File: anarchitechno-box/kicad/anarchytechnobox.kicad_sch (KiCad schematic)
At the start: 19 parts, among them J1 Conn_01x02, Q1 IRLZ44N, Q2 IRFS4310Z, U1 TC4426xOA, U2 ADuM1200AR, U4 LM7812_TO220, U5 L7805, U6 TME-0503S

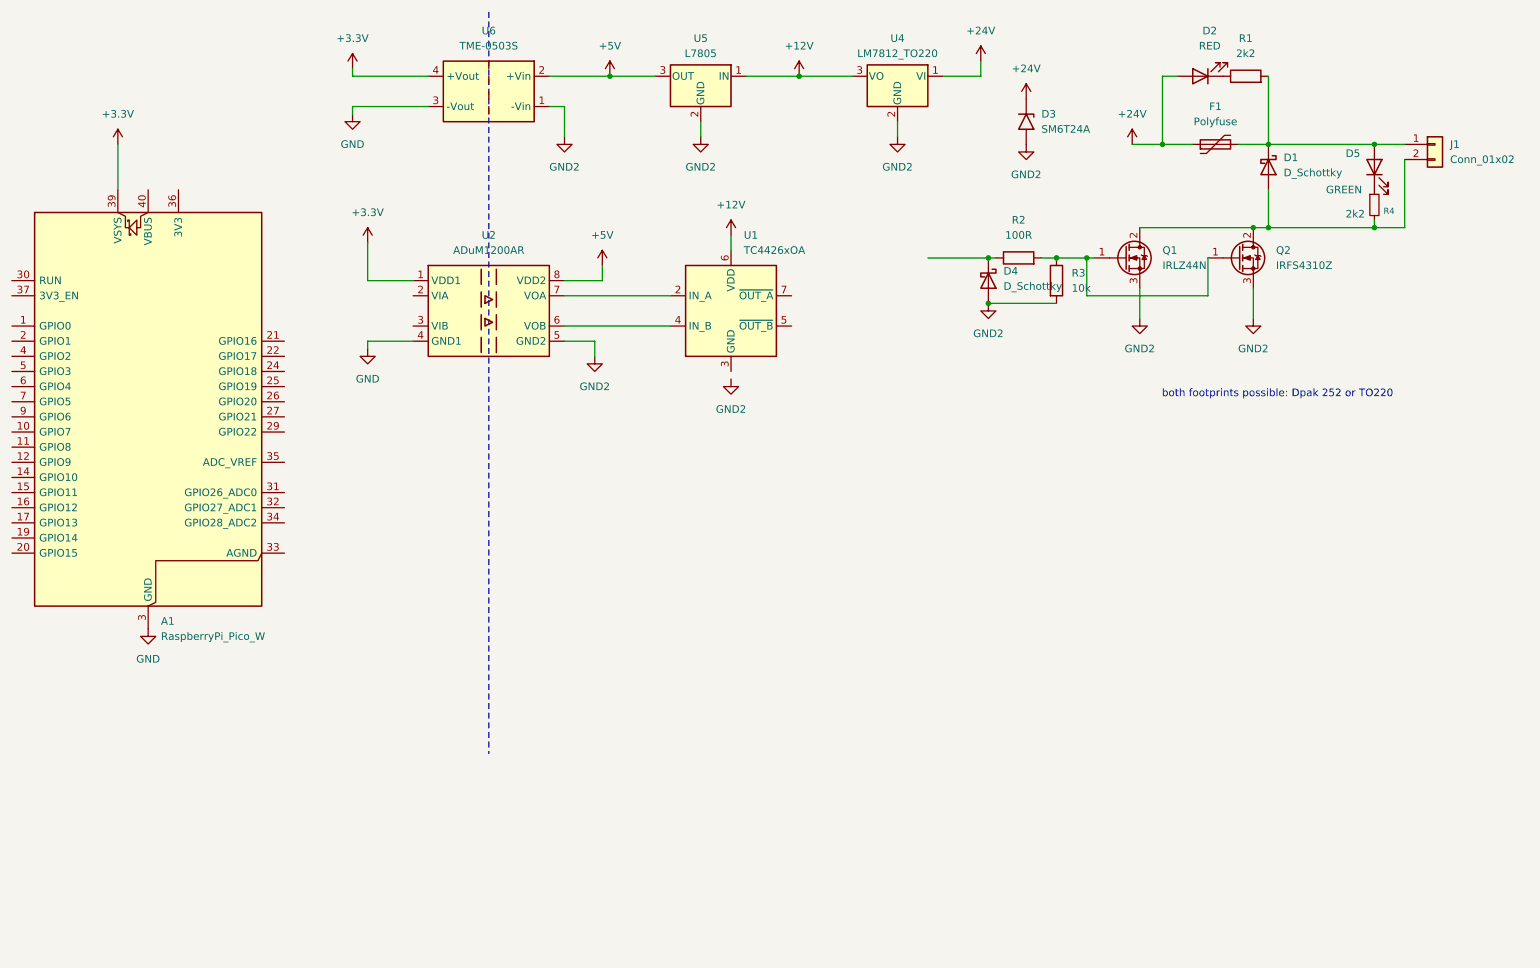
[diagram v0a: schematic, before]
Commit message: RP2350 initial commit
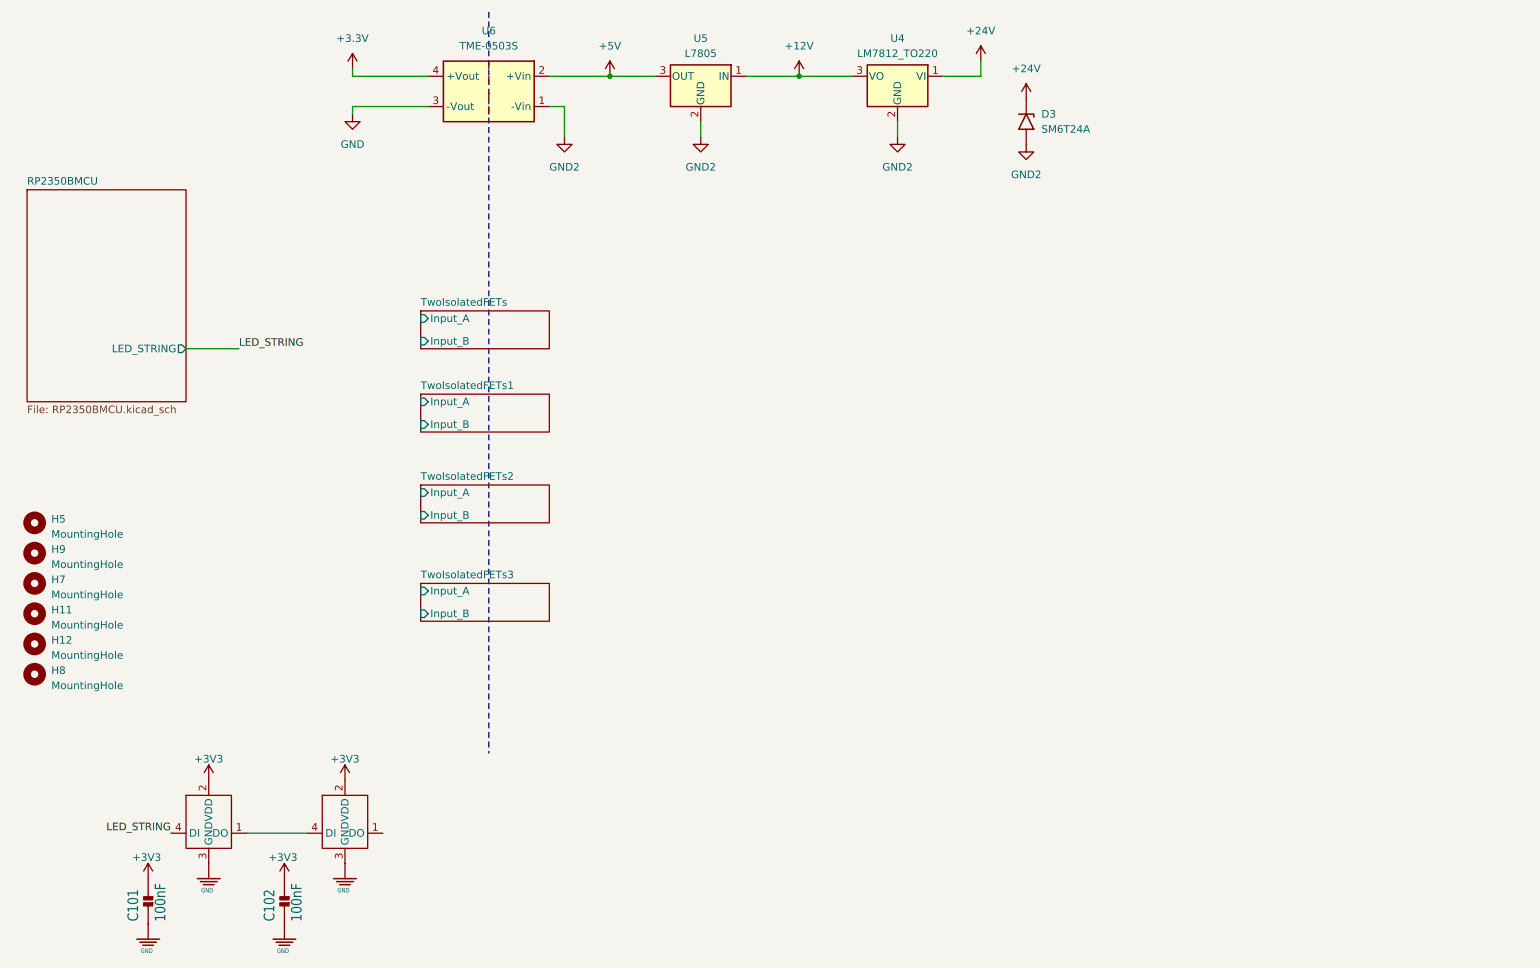
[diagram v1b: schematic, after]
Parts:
- removed A1: RaspberryPi_Pico_W, Module:RaspberryPi_Pico_W_SMD_HandSolder, symbol MCU_Module:RaspberryPi_Pico_W
- removed D1, D4: D_Schottky, symbol Device:D_Schottky
- removed D2: RED, symbol Device:LED
- removed D5: GREEN, symbol Device:LED
- removed F1: Polyfuse, symbol Device:Polyfuse
- removed J1: Conn_01x02, symbol Connector_Generic:Conn_01x02
- removed Q1: IRLZ44N, Package_TO_SOT_THT:TO-220-3_Vertical, symbol Transistor_FET:IRLZ44N
- removed Q2: IRFS4310Z, Package_TO_SOT_SMD:TO-263-2, symbol Transistor_FET:IRFS4310Z
- removed R1: 2k2, symbol Device:R
- removed R2: 100R, symbol Device:R
- removed R3: 10k, symbol Device:R
- removed R4: 2k2, symbol Device:R_Small
- removed U1: TC4426xOA, Package_SO:SOIC-8_3.9x4.9mm_P1.27mm, symbol Driver_FET:TC4426xOA
- removed U2: ADuM1200AR, Package_SO:SOIC-8_3.9x4.9mm_P1.27mm, symbol Isolator:ADuM1200AR
- added C101, C102: 100nF, Capacitor_SMD:C_0402_1005Metric, symbol TINRS - Wobbler (pico)sch-eagle-import:C-EUC0402
- added D1, D101: C5349953, TinyLEDs:XL-1010, symbol TinyLEDs:XL-1010
- added H11, H12, H5, H7, H8, H9: MountingHole, MountingHole:MountingHole_3.2mm_M3, symbol Mechanical:MountingHole
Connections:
- net GND: now also C101.1, C102.1, D1.3 (GND), D101.3 (GND)
- new net: D1.1 (DO), D101.4 (DI)
- new net +3V3: C101.2, C102.2, D1.2 (VDD), D101.2 (VDD)
- new net LED_STRING: D1.4 (DI)
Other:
- added sheet RP2350BMCU (RP2350BMCU.kicad_sch)
- added sheet TwoIsolatedFETs (TwoIsolatedFETs.kicad_sch)
- added sheet TwoIsolatedFETs1 (TwoIsolatedFETs.kicad_sch)
- added sheet TwoIsolatedFETs2 (TwoIsolatedFETs.kicad_sch)
- added sheet TwoIsolatedFETs3 (TwoIsolatedFETs.kicad_sch)
- note removed: "both footprints possible: Dpak 252 or TO220"

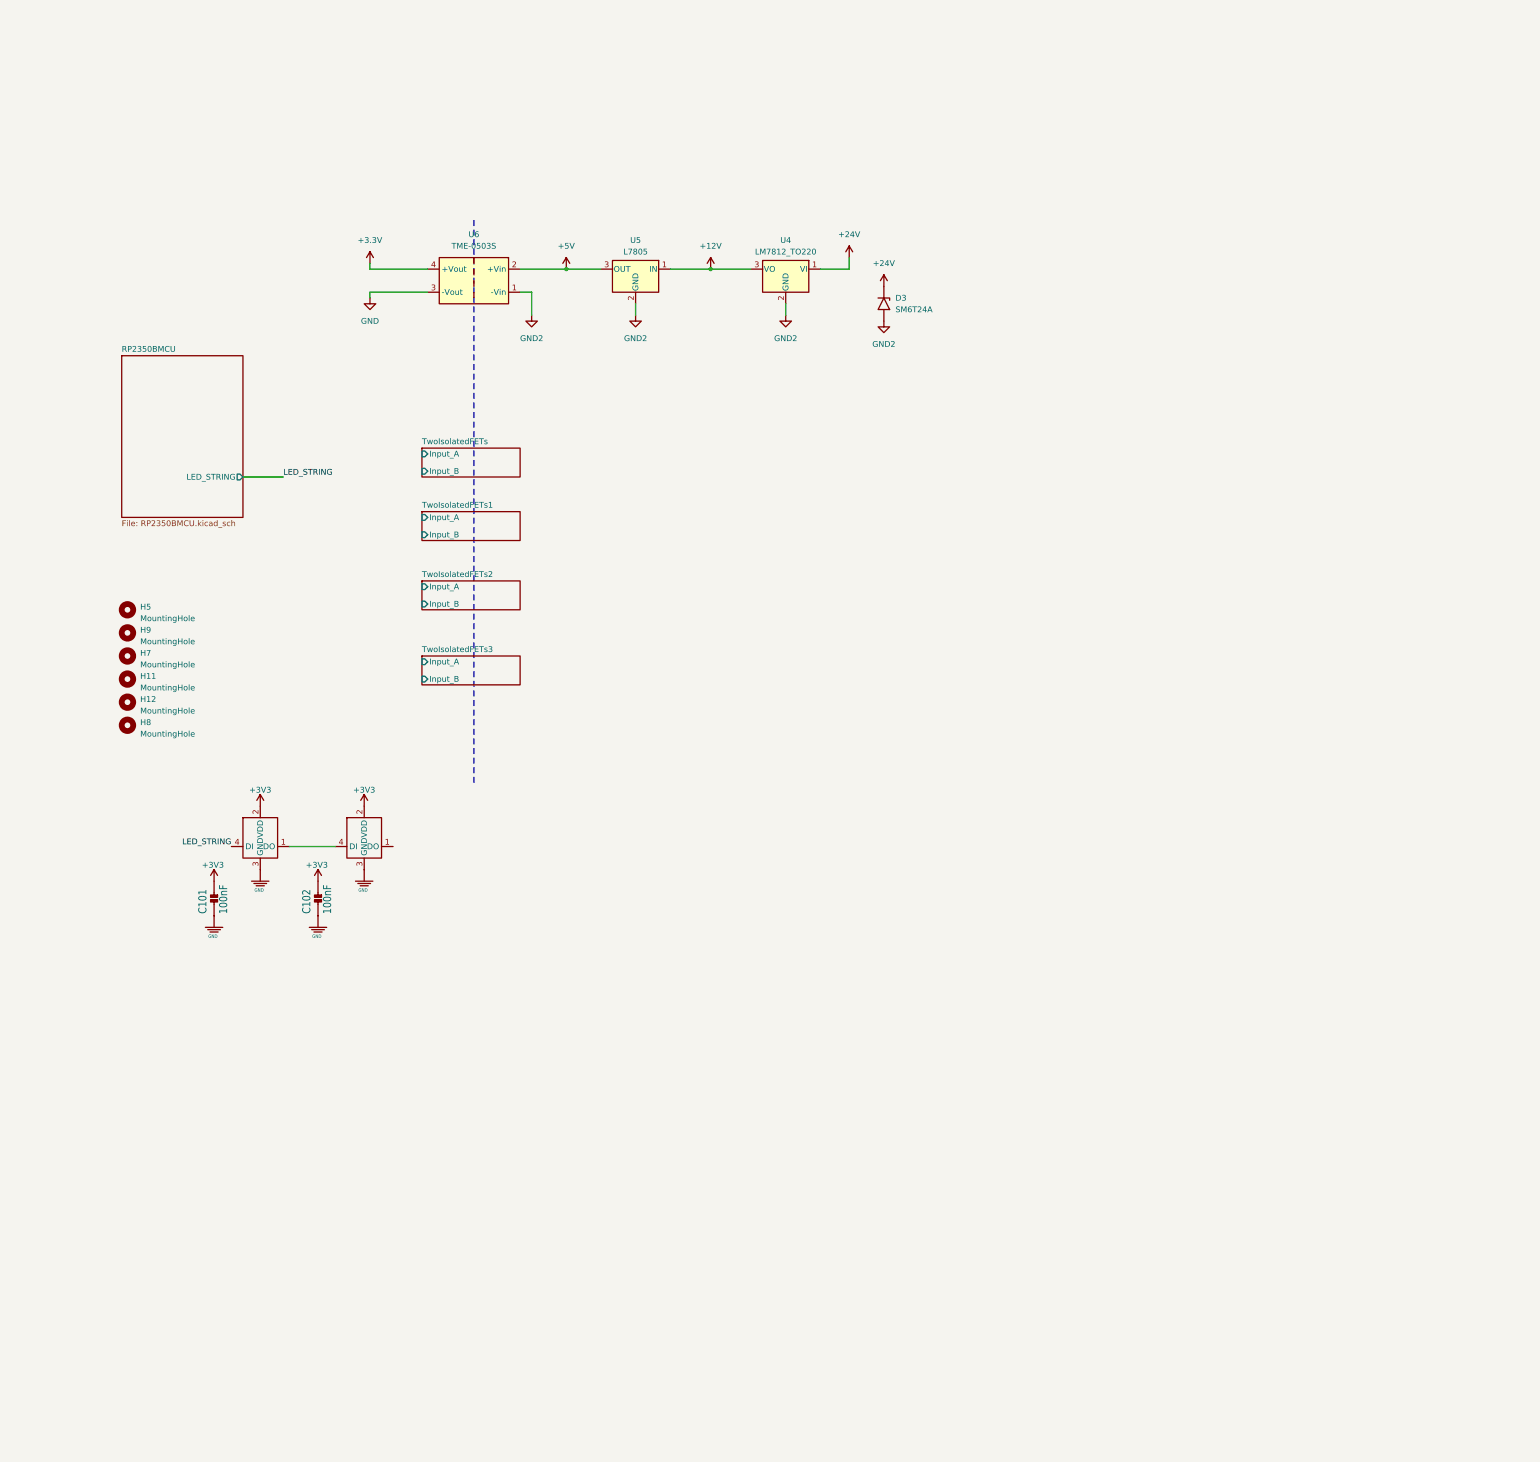
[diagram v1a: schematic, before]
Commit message: Large intermediate schematic push. Remaining todos are on frontpage.
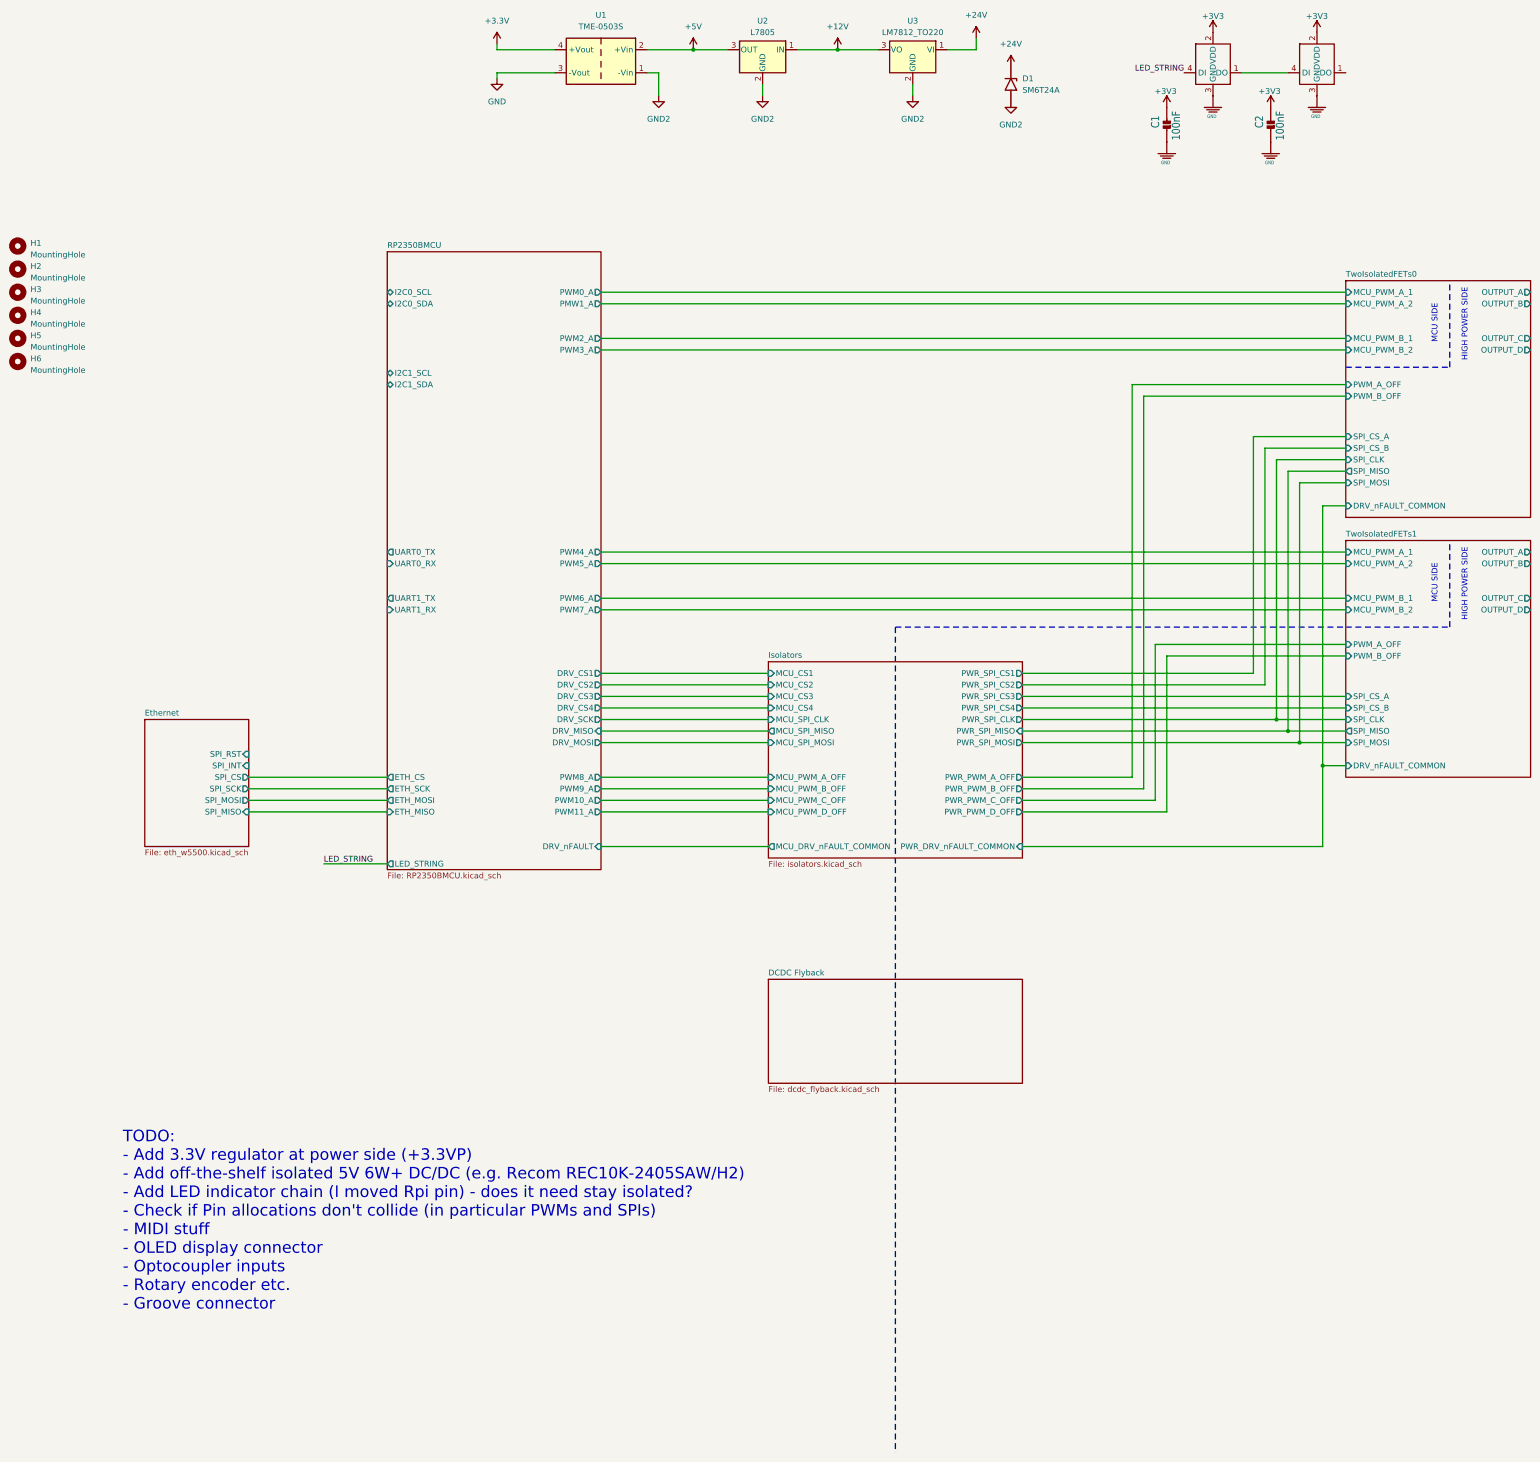
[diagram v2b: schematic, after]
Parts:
- renumbered C101 to C1, C102 to C2, D3 to D1, D1 to D2, D101 to D3, H5 to H1, H9 to H2, H7 to H3, H11 to H4, H12 to H5, H8 to H6, U6 to U1, U5 to U2, U4 to U3
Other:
- sheet TwoIsolatedFETs renamed TwoIsolatedFETs0
- removed sheet TwoIsolatedFETs2
- removed sheet TwoIsolatedFETs3
- added sheet DCDC Flyback (dcdc_flyback.kicad_sch)
- added sheet Ethernet (eth_w5500.kicad_sch)
- added sheet Isolators (isolators.kicad_sch)
- sheet RP2350BMCU ports: added DRV_CS1, DRV_CS2, DRV_CS3, DRV_CS4, DRV_MISO, DRV_MOSI, DRV_SCK, DRV_nFAULT, ETH_CS, ETH_MISO, ETH_MOSI, ETH_SCK, I2C0_SCL, I2C0_SDA, I2C1_SCL, I2C1_SDA, PMW1_A, PWM0_A, PWM10_A, PWM11_A, PWM2_A, PWM3_A, PWM4_A, PWM5_A, PWM6_A, PWM7_A, PWM8_A, PWM9_A, UART0_RX, UART0_TX, UART1_RX, UART1_TX; removed none
- sheet TwoIsolatedFETs0 ports: added DRV_nFAULT_COMMON, MCU_PWM_A_1, MCU_PWM_A_2, MCU_PWM_B_1, MCU_PWM_B_2, OUTPUT_A, OUTPUT_B, OUTPUT_C, OUTPUT_D, PWM_A_OFF, PWM_B_OFF, SPI_CLK, SPI_CS_A, SPI_CS_B, SPI_MISO, SPI_MOSI; removed Input_A, Input_B
- sheet TwoIsolatedFETs1 ports: added DRV_nFAULT_COMMON, MCU_PWM_A_1, MCU_PWM_A_2, MCU_PWM_B_1, MCU_PWM_B_2, OUTPUT_A, OUTPUT_B, OUTPUT_C, OUTPUT_D, PWM_A_OFF, PWM_B_OFF, SPI_CLK, SPI_CS_A, SPI_CS_B, SPI_MISO, SPI_MOSI; removed Input_A, Input_B
- note added: "HIGH POWER SIDE"
- note added: "MCU SIDE"
- note added: "TODO: - Add 3.3V regulator at power side (+3.3VP) - Add off-the-shelf isolated 5V 6W+ DC/DC (e.g. Recom REC10K-2405SAW/H2) - Add LED indicator chain (I moved Rpi pin) - does it need stay isolated? - Check if Pin allocations don't collide (in particular PWMs and SPIs) - MIDI stuff - OLED display connector - Optocoupler inputs - Rotary encoder etc. - Groove connector"
- moved on the sheet: C1, C2, D1, H1, H2, H3, H4, H5, H6, U1, U2, U3
